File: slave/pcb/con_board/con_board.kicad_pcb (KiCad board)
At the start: 2 copper layers, 43.2 x 43.2 mm, 8 parts, among them J1 CONN_01X01_FEMALE, J2 CONN_01X04_FEMALE, J3 CONN_01X04_FEMALE, J4 CONN_01X06, J5 CONN_01X06, J6 CONN_01X04, J7 CONN_01X04_FEMALE, J8 CONN_01X04_FEMALE

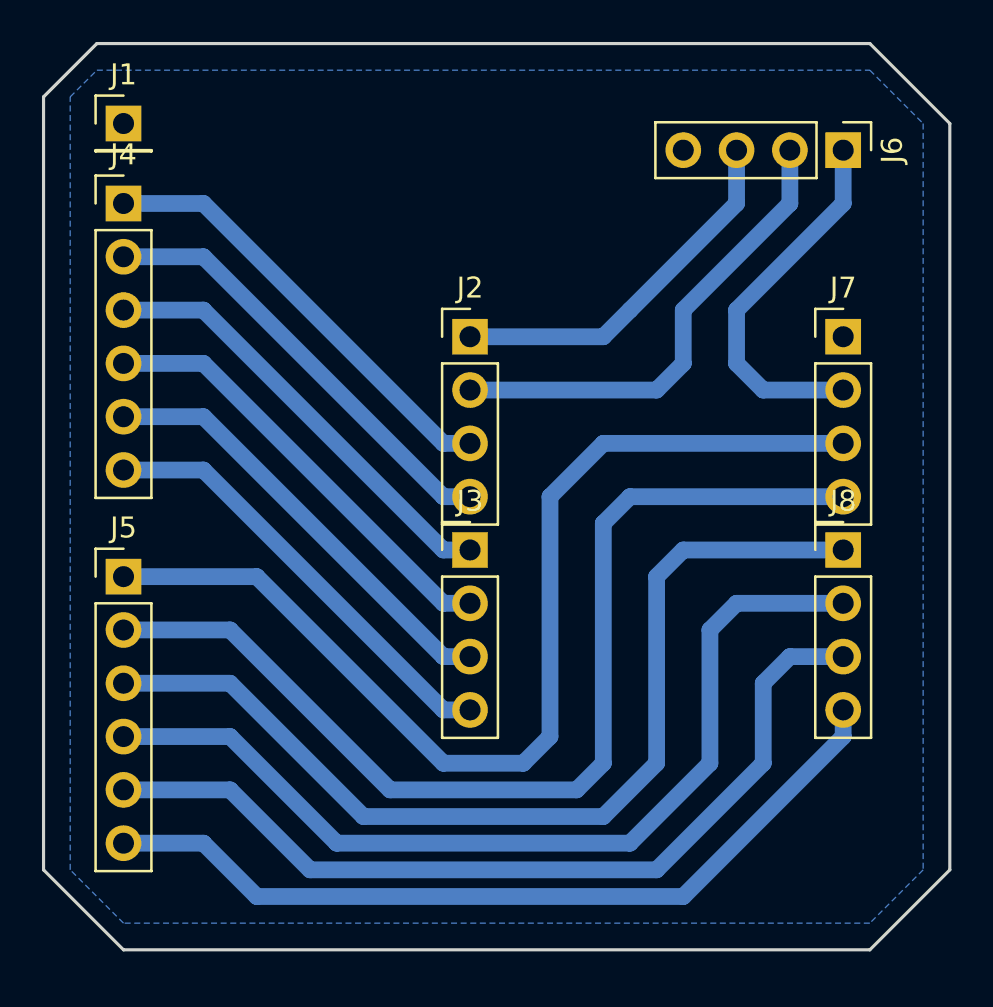
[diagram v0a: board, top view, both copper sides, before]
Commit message: pbc modifications
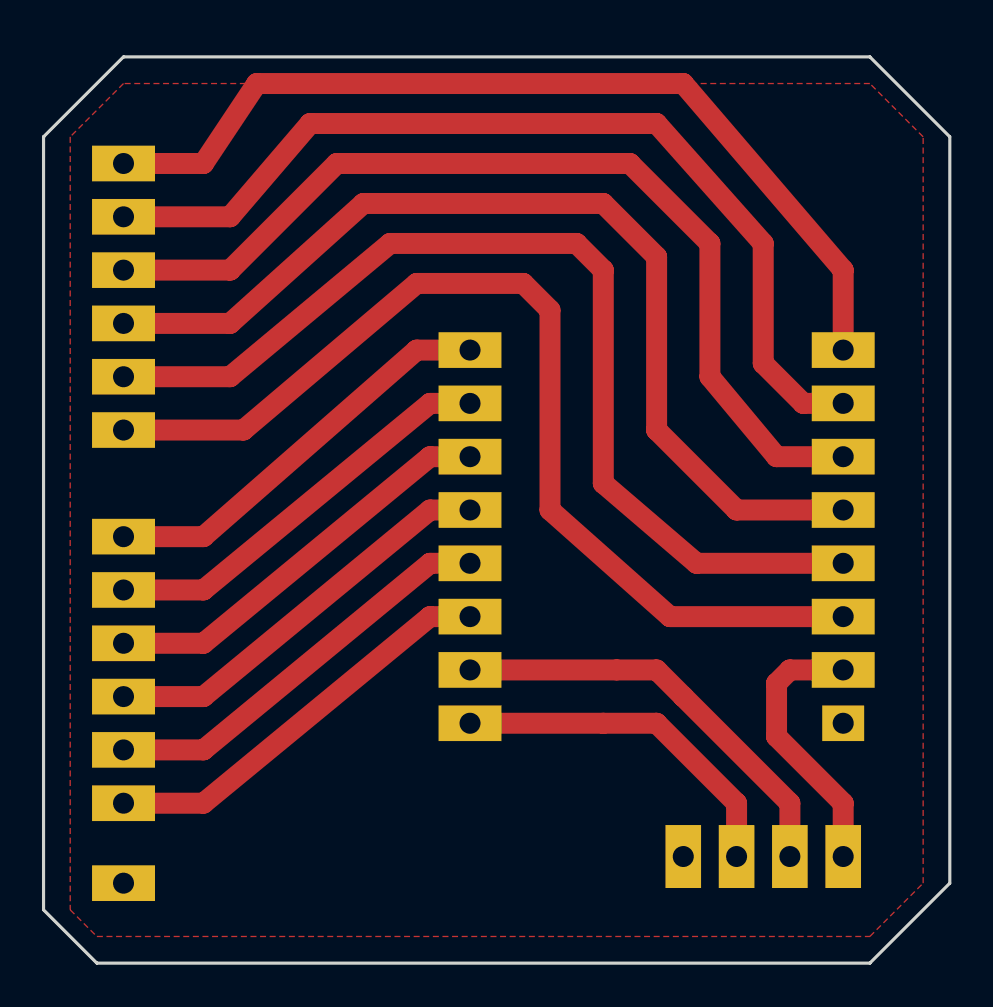
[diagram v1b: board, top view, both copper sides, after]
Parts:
- J1, J2, J3, J4, J5, J6, J7, J8: moved to B.Cu
- moved J1 36.2 mm to (139.7, 106.0)
- moved J6 33.7 mm to (174.0, 104.8), turned to 90 degrees
- moved J4 28.6 mm to (139.7, 102.2)
- moved J2 18.4 mm to (156.2, 98.4)
- moved J7 18.4 mm to (174.0, 98.4)
- moved J5 6.98 mm to (139.7, 84.5)
- moved J3 1.91 mm to (156.2, 88.3)
- moved J8 1.91 mm to (174.0, 88.3)
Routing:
- net 5V: track 17.9 -> 13.0 mm
- net Net-(J5-Pad6): track 39.8 -> 44.2 mm
- net Net-(J5-Pad5): track 42.3 -> 45.4 mm
- net SDA: track 23.0 -> 20.4 mm
- net Net-(J5-Pad1): track 51.0 -> 48.8 mm
- net Net-(J3-Pad3): track 21.2 -> 19.7 mm
- net Net-(J3-Pad1): track 21.2 -> 19.7 mm
- net Net-(J2-Pad3): track 21.2 -> 19.7 mm
- net Net-(J2-Pad4): track 21.2 -> 19.7 mm
- net Net-(J3-Pad2): track 21.2 -> 19.7 mm
- net Net-(J3-Pad4): track 21.2 -> 19.9 mm
- net Net-(J5-Pad4): track 44.8 -> 46.1 mm
- net Net-(J5-Pad2): track 49.9 -> 48.7 mm
- net SCL: track 17.9 -> 16.8 mm
- added copper zone on F.Cu, net GND
- removed copper zone on B.Cu, net GND
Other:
- outline, holes or cut-outs redrawn
